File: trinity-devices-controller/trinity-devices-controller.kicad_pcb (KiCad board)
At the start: 4 copper layers, 90 parts, among them IC1 LM25145RGYR, IC2 MCP2562, J1 xh2pin, J10 xh2pin, J11 Conn_01x03, J12 Conn_01x03, J13 Conn_01x03, J2 xh2pin, J3 Conn_01x01_Pin, J4 Conn_01x01_Pin, J5 Conn_01x04, J6 Conn_01x04, J7 Conn_01x04_Pin, J8 Conn_01x04, J9 xh2pin, Q1 IRFML8244TRPBFTR, Q2 IRFML8244TRPBFTR, Q3 TPH7R506NH,L1Q, Q4 TPH2R306NH1,LQ, Q5 IRFML8244TRPBFTR, Q6 IRFML8244TRPBFTR, SW1 SW_Push, U1 TLP293-4, U3 STM32G431K8Tx, U4 NJM12888F33, U6 NJM7805SDL1, U8 ISO6540FQDBQRQ1

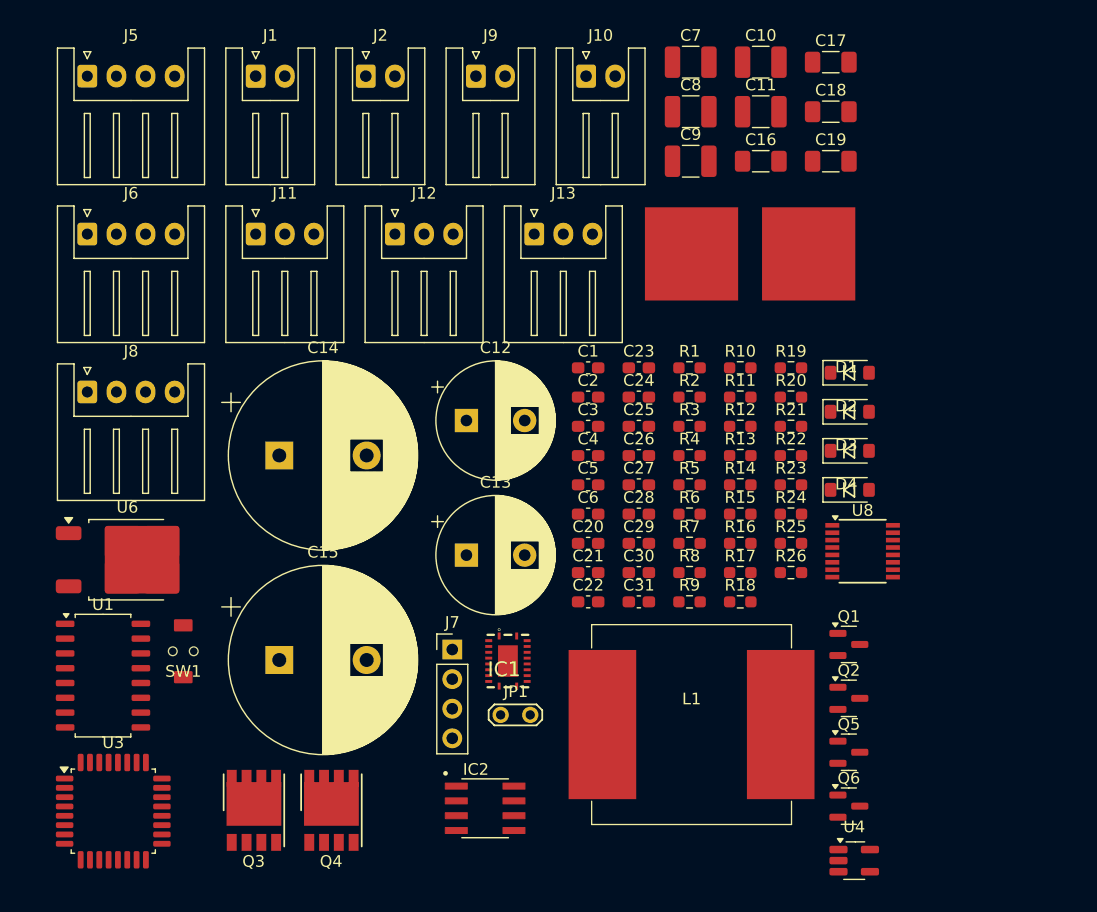
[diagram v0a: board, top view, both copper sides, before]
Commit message: 配置、配線完了
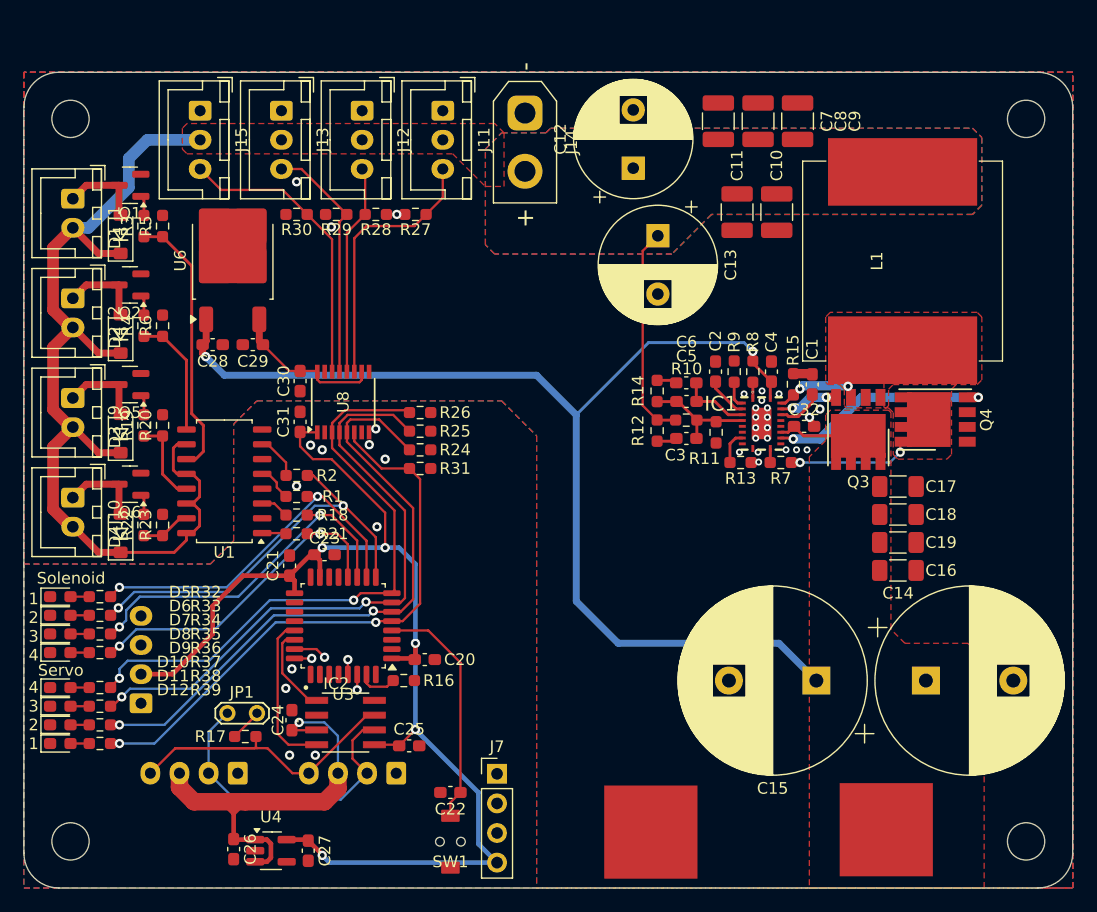
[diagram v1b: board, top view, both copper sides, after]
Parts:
- added C32: 0.1uf, Capacitor_SMD:C_0603_1608Metric_Pad1.08x0.95mm_HandSolder, F.Cu at (82.0, 45.4)
- added D10: LED, LED_SMD:LED_0603_1608Metric_Pad1.05x0.95mm_HandSolder, F.Cu at (18.1, 69.4)
- added D11: LED, LED_SMD:LED_0603_1608Metric_Pad1.05x0.95mm_HandSolder, F.Cu at (18.1, 71.0)
- added D12: LED, LED_SMD:LED_0603_1608Metric_Pad1.05x0.95mm_HandSolder, F.Cu at (18.1, 72.6)
- added D5: LED, LED_SMD:LED_0603_1608Metric_Pad1.05x0.95mm_HandSolder, F.Cu at (18.1, 60.0)
- added D6: LED, LED_SMD:LED_0603_1608Metric_Pad1.05x0.95mm_HandSolder, F.Cu at (18.1, 61.6)
- added D7: LED, LED_SMD:LED_0603_1608Metric_Pad1.05x0.95mm_HandSolder, F.Cu at (18.1, 63.2)
- added D8: LED, LED_SMD:LED_0603_1608Metric_Pad1.05x0.95mm_HandSolder, F.Cu at (18.1, 64.8)
- added D9: LED, LED_SMD:LED_0603_1608Metric_Pad1.05x0.95mm_HandSolder, F.Cu at (18.1, 67.8)
- added J14: Conn_01x02, Connector_AMASS:AMASS_XT30UPB-M_1x02_P5.0mm_Vertical, F.Cu at (58.0, 18.5)
- added J15: Conn_01x03, Connector_JST:JST_XH_B3B-XH-A_1x03_P2.50mm_Vertical, F.Cu at (30.1, 18.3)
- added R27: 10k, Resistor_SMD:R_0603_1608Metric_Pad0.98x0.95mm_HandSolder, F.Cu at (48.6, 27.2)
- added R28: 10k, Resistor_SMD:R_0603_1608Metric_Pad0.98x0.95mm_HandSolder, F.Cu at (45.2, 27.2)
- added R29: 10k, Resistor_SMD:R_0603_1608Metric_Pad0.98x0.95mm_HandSolder, F.Cu at (41.8, 27.2)
- added R30: 10k, Resistor_SMD:R_0603_1608Metric_Pad0.98x0.95mm_HandSolder, F.Cu at (38.4, 27.2)
- added R31: 10k, Resistor_SMD:R_0603_1608Metric_Pad0.98x0.95mm_HandSolder, F.Cu at (49.0, 49.0)
- added R32: 1k, Resistor_SMD:R_0603_1608Metric_Pad0.98x0.95mm_HandSolder, F.Cu at (21.5, 60.0)
- added R33: 1k, Resistor_SMD:R_0603_1608Metric_Pad0.98x0.95mm_HandSolder, F.Cu at (21.5, 61.6)
- added R34: 1k, Resistor_SMD:R_0603_1608Metric_Pad0.98x0.95mm_HandSolder, F.Cu at (21.5, 63.2)
- added R35: 1k, Resistor_SMD:R_0603_1608Metric_Pad0.98x0.95mm_HandSolder, F.Cu at (21.5, 64.8)
- added R36: 1k, Resistor_SMD:R_0603_1608Metric_Pad0.98x0.95mm_HandSolder, F.Cu at (21.5, 67.8)
- added R37: 1k, Resistor_SMD:R_0603_1608Metric_Pad0.98x0.95mm_HandSolder, F.Cu at (21.5, 69.4)
- added R38: 1k, Resistor_SMD:R_0603_1608Metric_Pad0.98x0.95mm_HandSolder, F.Cu at (21.5, 71.0)
- added R39: 1k, Resistor_SMD:R_0603_1608Metric_Pad0.98x0.95mm_HandSolder, F.Cu at (21.5, 72.6)
- added REF**: MountingHole_3.2mm_M3, MountingHole:MountingHole_3.2mm_M3, F.Cu at (19.0, 19.0)
- added REF**: MountingHole_3.2mm_M3, MountingHole:MountingHole_3.2mm_M3, F.Cu at (19.0, 81.0)
- added REF**: MountingHole_3.2mm_M3, MountingHole:MountingHole_3.2mm_M3, F.Cu at (101.0, 19.0)
- added REF**: MountingHole_3.2mm_M3, MountingHole:MountingHole_3.2mm_M3, F.Cu at (101.0, 81.0)
- J1, J10, J2, J9: footprint Connector_JST:JST_XH_S2B-XH-A_1x02_P2.50mm_Horizontal -> Connector_JST:JST_XH_B2B-XH-A_1x02_P2.50mm_Vertical
- J11, J12, J13: footprint Connector_JST:JST_XH_S3B-XH-A_1x03_P2.50mm_Horizontal -> Connector_JST:JST_XH_B3B-XH-A_1x03_P2.50mm_Vertical
- J5, J6, J8: moved to B.Cu
- moved Q1 73.2 mm to (24.1, 24.7), turned to 180 degrees
- moved Q2 71.2 mm to (24.1, 33.2), turned to 180 degrees
- moved Q5 69.3 mm to (24.1, 41.8), turned to 180 degrees
- moved Q6 67.6 mm to (24.1, 50.4), turned to 180 degrees
- moved D1 63.3 mm to (23.3, 29.2), turned to 90 degrees
- moved D2 62.6 mm to (23.3, 37.8), turned to 90 degrees
- moved D4 62.4 mm to (23.3, 54.9), turned to 90 degrees
- moved D3 62.3 mm to (23.3, 46.3), turned to 90 degrees
- moved Q4 61.7 mm to (93.2, 44.8), turned to 90 degrees
- moved Q3 61.3 mm to (86.6, 45.6), turned to 180 degrees
- moved J5 61.2 mm to (33.4, 75.2), turned to 180 degrees
- moved C14 58.8 mm to (92.4, 67.2)
- moved J10 57.0 mm to (19.2, 51.5), turned to -90 degrees
- moved R22 55.8 mm to (25.3, 53.9), turned to 90 degrees
- moved R19 55.7 mm to (25.3, 45.3), turned to 90 degrees
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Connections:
- C6 pad 1: Net-(C6-Pad1) -> Net-(IC1-COMP)
- C6 pad 2: Net-(IC1-FB) -> Net-(C6-Pad2)
- J11 pad 2: PWM1 -> +12V
- J11 pad 3: +12V -> PWM1
- J12 pad 2: PWM2 -> +12V
- J12 pad 3: +12V -> PWM2
- J13 pad 2: PWM3 -> +12V
- J13 pad 3: +12V -> PWM3
- R14 pad 1: Net-(IC1-COMP) -> Net-(C6-Pad2)
- R14 pad 2: Net-(C6-Pad1) -> Net-(IC1-FB)
- R24 pad 1: TIM2_CH3 -> TIM2_CH2
- R25 pad 1: TIM2_CH2 -> TIM2_CH3
- R26 pad 1: TIM2_CH1 -> TIM2_CH4
- U1 pad 1: Net-(R1-Pad2) -> Net-(R21-Pad2)
- U1 pad 11: Net-(R19-Pad1) -> Net-(R3-Pad1)
- U1 pad 13: Net-(R4-Pad1) -> Net-(R19-Pad1)
- U1 pad 15: Net-(R3-Pad1) -> Net-(R22-Pad1)
- U1 pad 3: Net-(R2-Pad2) -> Net-(R18-Pad2)
- U1 pad 5: Net-(R18-Pad2) -> Net-(R1-Pad2)
- U1 pad 7: Net-(R21-Pad2) -> Net-(R2-Pad2)
- U1 pad 9: Net-(R22-Pad1) -> Net-(R4-Pad1)
- U3 pad 10: IN2 -> IN1
- U3 pad 8: unconnected-(U3-PA3-Pad8) -> TIM2_CH4
- U3 pad 9: IN1 -> IN2
- U8 pad 11: unconnected-(U8-OUTD-Pad11) -> PWM1
- U8 pad 12: PWM3 -> PWM2
- U8 pad 13: PWM2 -> PWM3
- U8 pad 14: PWM1 -> PWM4
- U8 pad 3: TIM2_CH1 -> TIM2_CH4
- U8 pad 4: TIM2_CH2 -> TIM2_CH3
- U8 pad 5: TIM2_CH3 -> TIM2_CH2
- U8 pad 6: unconnected-(U8-IND-Pad6) -> TIM2_CH1
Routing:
- net VCC: track 0.00 -> 106.7 mm, vias 0 -> 2
- net +3.3V: track 0.00 -> 104.2 mm, vias 0 -> 5
- net +12V: track 0.00 -> 103.5 mm
- net TIM2_CH2: track 0.00 -> 54.5 mm, vias 0 -> 2
- net TIM2_CH3: track 0.00 -> 53.4 mm, vias 0 -> 2
- net TIM2_CH4: track 0.00 -> 52.1 mm, vias 0 -> 2
- net TIM2_CH1: track 0.00 -> 50.0 mm, vias 0 -> 2
- net +5V: track 0.00 -> 40.7 mm, vias 0 -> 1
- net IN2: track 0.00 -> 35.4 mm, vias 0 -> 2
- net IN1: track 0.00 -> 31.5 mm, vias 0 -> 2
- net CANH: track 0.00 -> 31.1 mm
- net IN3: track 0.00 -> 31.0 mm, vias 0 -> 2
- net IN4: track 0.00 -> 28.9 mm, vias 0 -> 2
- net CANL: track 0.00 -> 26.9 mm
- net SWCLK: track 0.00 -> 26.0 mm, vias 0 -> 1
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- added copper zone on B.Cu, net +12V
- added copper zone on F.Cu, net +12V
- added copper zone on In1.Cu, net +12V
- added copper zone on In2.Cu, net +12V
- added copper zone on B.Cu, net GND
- added copper zone on F.Cu, net GND
- added copper zone on In1.Cu, net GND
- added copper zone on In2.Cu, net GND
- added copper zone on B.Cu, net GNDD
- added copper zone on F.Cu, net GNDD
- added copper zone on In1.Cu, net GNDD
- added copper zone on In2.Cu, net GNDD
- added copper zone on F.Cu, net Net-(IC1-SW)
- added copper zone on F.Cu, net VCC
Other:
- board outline added: 90 x 70 mm
- board text added: "1 2 3 4"
- board text added: "4 3 2 1"
- board text added: "Servo"
- board text added: "Solenoid"
